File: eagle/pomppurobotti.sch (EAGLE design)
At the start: 3 parts

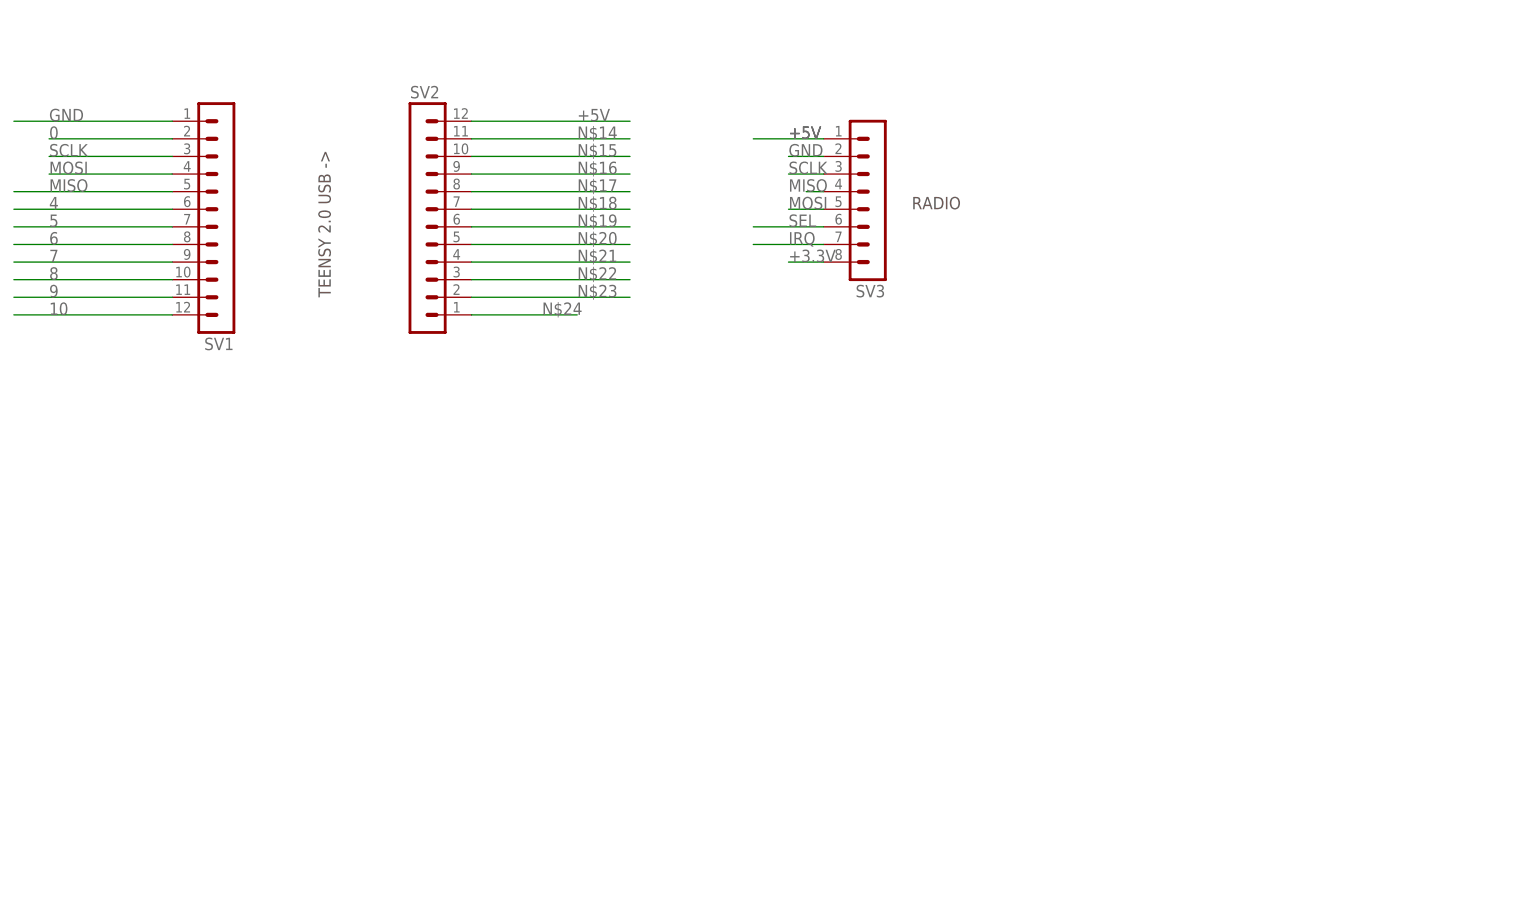
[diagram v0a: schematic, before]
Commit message: First version of PCB
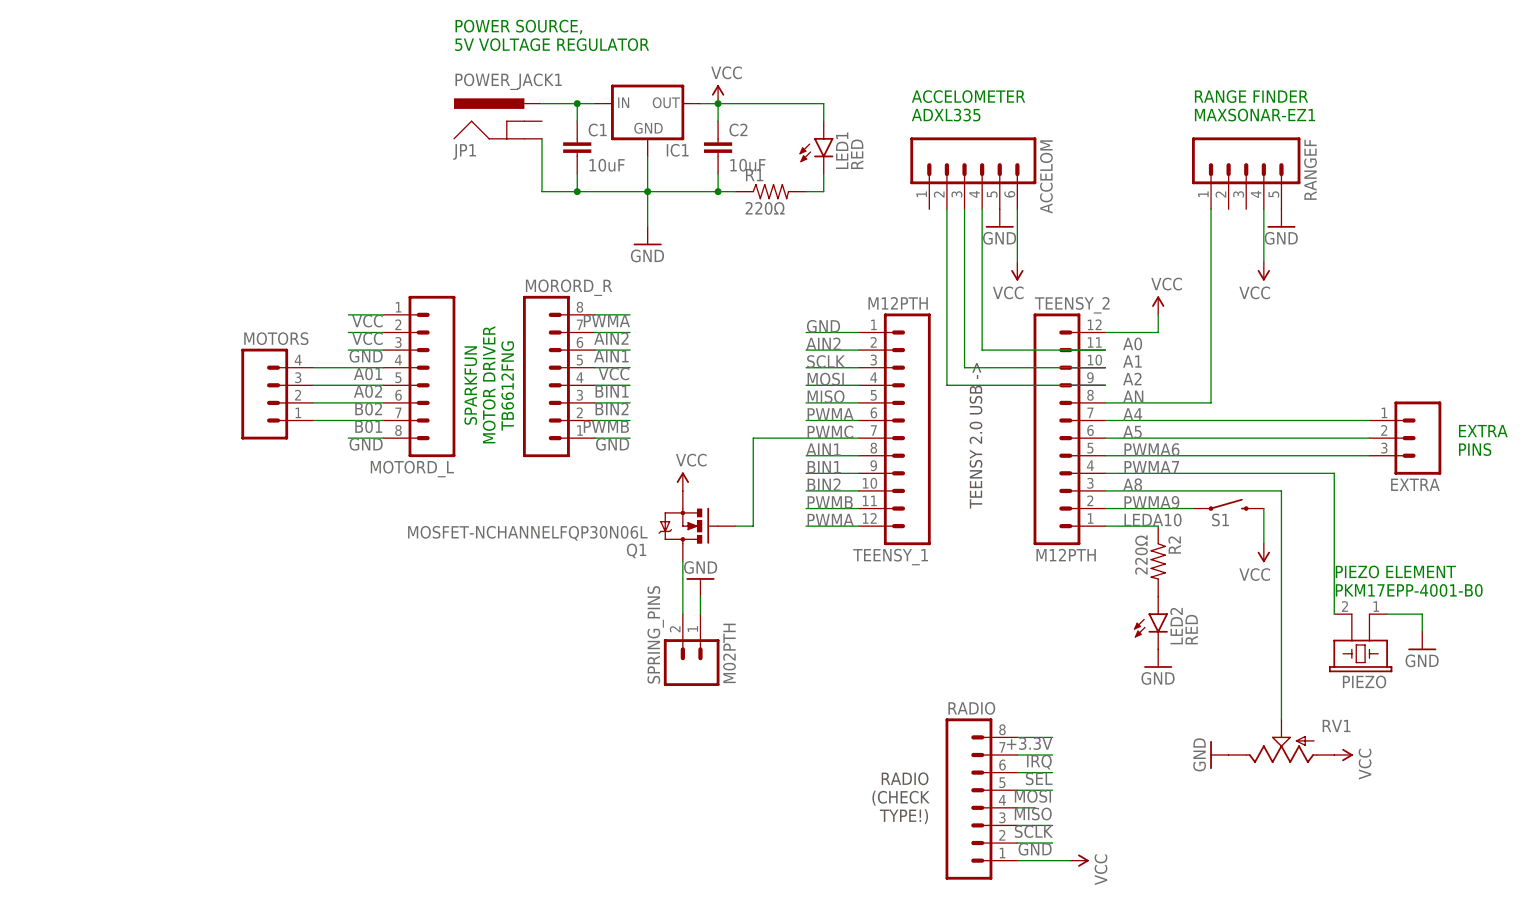
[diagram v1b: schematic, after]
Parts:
- removed SV1, SV2: (no value), con-lstb:MA12-1
- removed SV3: (no value), con-lstb:MA08-1
- added ACCELOM: (no value), SparkFun-Connectors:M06SILK_FEMALE_PTH
- added C1, C2: 10uF, SparkFun-Capacitors:CAPPTH
- added EXTRA: (no value), SparkFun-Connectors:M03PTH
- added IC1: (no value), SparkFun-PowerIC:V_REG_78XX-TO-220
- added JP1: POWER_JACK1, SparkFun-Connectors:POWER_JACK1
- added LED1, LED2: RED, SparkFun-LED:LED5MM
- added MORORD_R, MOTORD_L: (no value), SparkFun-Connectors:M08LONGPADS
- added MOTORS: (no value), SparkFun-Connectors:M04PTH
- added PIEZO: EFBAA40D101, buzzer:EFBAA40D101
- added Q1: MOSFET-NCHANNELFQP30N06L, SparkFun-DiscreteSemi:MOSFET-NCHANNELFQP30N06L
- added R1, R2: 220Ω, SparkFun-Resistors:RESISTORAXIAL-0.3
- added RADIO: (no value), SparkFun-Connectors:M08
- added RANGEF: (no value), SparkFun-Connectors:M05PTH
- added RV1: (no value), SparkFun-Electromechanical:POTTRIM
- added S1: SWITCH-MOMENTARY-2PTH, SparkFun-Electromechanical:SWITCH-MOMENTARY-2PTH
- added SPRING_PINS: M02PTH, SparkFun-Connectors:M02PTH
- added TEENSY_1, TEENSY_2: M12PTH, SparkFun-Connectors:M12PTH
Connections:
- removed net +5V: SV2.12, SV3.1
- removed net 0: SV1.2
- removed net 10: SV1.12
- removed net 4: SV1.6
- removed net 5: SV1.7
- removed net 6: SV1.8
- removed net 7: SV1.9
- removed net 8: SV1.10
- removed net 9: SV1.11
- removed net N$14: SV2.11
- removed net N$15: SV2.10
- removed net N$16: SV2.9
- removed net N$17: SV2.8
- removed net N$18: SV2.7
- removed net N$19: SV2.6
- removed net N$20: SV2.5
- removed net N$21: SV2.4
- removed net N$22: SV2.3
- removed net N$23: SV2.2
- removed net N$24: SV2.1
- new net A0: ACCELOM.2, TEENSY_2.9
- new net A01: MOTORD_L.4, MOTORS.4
- new net A02: MOTORD_L.5, MOTORS.3
- new net A1: ACCELOM.3, TEENSY_2.10
- new net A2: ACCELOM.4, TEENSY_2.11
- new net A4: EXTRA.1, TEENSY_2.7
- new net A5: EXTRA.2, TEENSY_2.6
- new net A8: RV1.S, TEENSY_2.3
- new net AIN1: MORORD_R.6, TEENSY_1.8
- new net AIN2: MORORD_R.7, TEENSY_1.2
- new net AN: RANGEF.1, TEENSY_2.8
- new net B01: MOTORD_L.7, MOTORS.1
- new net B02: MOTORD_L.6, MOTORS.2
- new net BIN1: MORORD_R.4, TEENSY_1.9
- new net BIN2: MORORD_R.3, TEENSY_1.10
- new net LEDA10: R2.1, TEENSY_2.1
- new net N$2: LED1.C, R1.2
- new net N$3: C1.1, IC1.IN, JP1.PWR
- new net N$4: LED2.A, R2.2
- new net N$5: Q1.D, SPRING_PINS.2
- new net PWMA: MORORD_R.8, TEENSY_1.12, TEENSY_1.6
- new net PWMA6: EXTRA.3, TEENSY_2.5
- new net PWMA7: PIEZO.2, TEENSY_2.4
- new net PWMA9: S1.1, TEENSY_2.2
- new net PWMB: MORORD_R.2, TEENSY_1.11
- new net PWMC: Q1.G, TEENSY_1.7
- new net VCC: ACCELOM.6, C2.1, IC1.OUT, LED1.A, MORORD_R.5, MOTORD_L.1, MOTORD_L.2, Q1.S, RADIO.1, RANGEF.4, RV1.A, S1.2, TEENSY_2.12
- net +3.3V: now also RADIO.8; no longer SV3.8
- net GND: now also ACCELOM.5, C1.2, C2.2, IC1.GND, JP1.GND, LED2.C, MORORD_R.1, MOTORD_L.3, MOTORD_L.8, PIEZO.1, R1.1, RADIO.2, RANGEF.5, RV1.E, SPRING_PINS.1, TEENSY_1.1; no longer SV1.1, SV3.2
- net IRQ: now also RADIO.7; no longer SV3.7
- net MISO: now also RADIO.4, TEENSY_1.5; no longer SV1.5, SV3.4
- net MOSI: now also RADIO.5, TEENSY_1.4; no longer SV1.4, SV3.5
- net SCLK: now also RADIO.3, TEENSY_1.3; no longer SV1.3, SV3.3
- net SEL: now also RADIO.6; no longer SV3.6
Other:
- note added: "ACCELOMETER ADXL335"
- note added: "EXTRA PINS"
- note added: "PIEZO ELEMENT PKM17EPP-4001-B0"
- note added: "POWER SOURCE, 5V VOLTAGE REGULATOR"
- note added: "RADIO (CHECK TYPE!)"
- note added: "RANGE FINDER MAXSONAR-EZ1"
- note added: "SPARKFUN MOTOR DRIVER TB6612FNG"
- note removed: "RADIO"
